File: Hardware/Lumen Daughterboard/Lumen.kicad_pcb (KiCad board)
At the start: 2 copper layers, 18 x 11 mm, 16 parts, among them J5 PRT-14417, U1 ATtiny1617-M, U2 BNO055

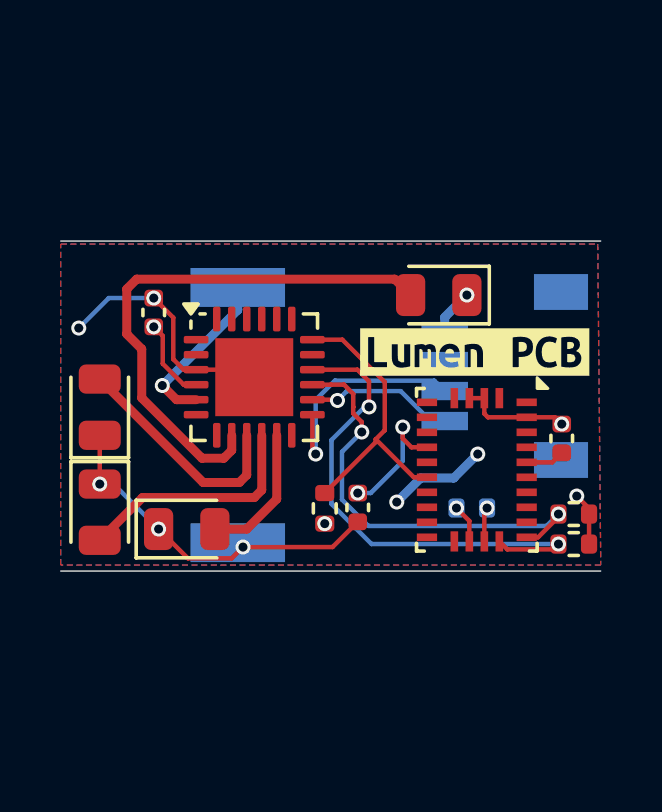
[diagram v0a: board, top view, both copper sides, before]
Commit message: Lumen :D
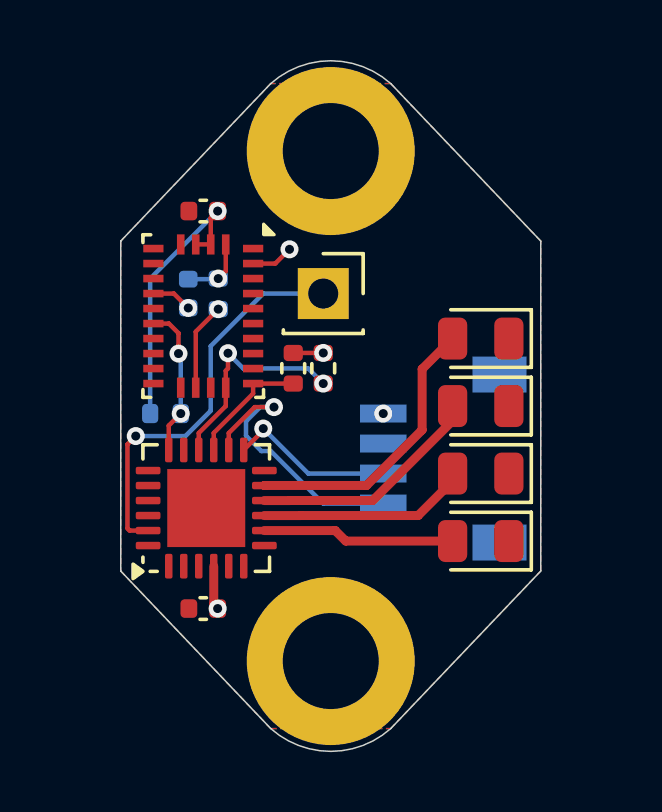
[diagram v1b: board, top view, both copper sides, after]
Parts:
- removed BZ1: Buzzer, User:CPT-9019A_CUD
- removed kibuzzard-68C38C57: G***, kibuzzard-68C38C57
- added J1: Conn_01x01_Socket, Connector_PinSocket_2.54mm:PinSocket_1x01_P2.54mm_Vertical, F.Cu at (112.8, 31.8)
- added REF**: MountingHole_3.2mm_M3_DIN965_Pad, MountingHole:MountingHole_3.2mm_M3_DIN965_Pad, F.Cu at (113.0, 44.0)
- added REF**: MountingHole_3.2mm_M3_DIN965_Pad, MountingHole:MountingHole_3.2mm_M3_DIN965_Pad, F.Cu at (113.0, 27.0)
- C3, R1: moved to B.Cu
- moved C2 14.2 mm to (108.8, 29.0), turned to 0 degrees
- moved D3 13.2 mm to (118.0, 35.5), turned to 180 degrees
- moved D2 12.9 mm to (118.0, 37.8), turned to 180 degrees
- moved D4 11.7 mm to (118.0, 33.2), turned to 180 degrees
- moved R4 11.1 mm to (109.2, 31.8), turned to 90 degrees
- moved R2 10.5 mm to (111.8, 34.2), turned to 90 degrees
- moved U2 10.5 mm to (108.8, 32.5)
- moved R3 10.2 mm to (112.8, 34.2), turned to 90 degrees
- moved C1 10.0 mm to (108.8, 42.2), turned to 0 degrees
- moved C3 9.10 mm to (108.2, 31.8), turned to -90 degrees
- moved D1 8.32 mm to (118.0, 40.0)
- moved R1 6.18 mm to (107.5, 35.8), turned to 180 degrees
- moved U1 4.65 mm to (108.8, 38.9), turned to 90 degrees
- moved J5 3.23 mm to (117.2, 37.2)
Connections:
- U1 pad 5: Net-(BZ1-+) -> unconnected-(U1-PA4-Pad5)
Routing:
- net GND: track 27.2 -> 2.25 mm, vias 9 -> 2
- net /UPDI: track 0.00 -> 13.4 mm, vias 0 -> 1
- net Net-(D1-A): track 18.1 -> 6.42 mm
- net /SDA: track 14.6 -> 4.09 mm, vias 2 -> 0
- net /SCL: track 17.0 -> 7.22 mm
- net Net-(BZ1-+): track 5.64 -> 0.00 mm, vias 1 -> 0
- net +V: track 8.26 -> 13.3 mm
- net Net-(D4-A): track 4.60 -> 9.49 mm
- net /~{BNO_RST}: track 9.76 -> 5.06 mm, vias 0 -> 2
- net /TX: track 4.96 -> 9.55 mm
- net Net-(U2-CAP): track 4.38 -> 1.36 mm, vias 2 -> 1
- net /RX: track 7.88 -> 5.60 mm
- net Net-(U2-COM3): track 1.29 -> 2.93 mm
- net Net-(D2-A): track 7.76 -> 7.00 mm
- net Net-(D3-A): track 7.92 -> 7.36 mm
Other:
- board size 18 x 11 mm -> 14 x 23 mm
